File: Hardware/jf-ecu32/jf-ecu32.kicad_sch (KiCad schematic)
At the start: 41 parts, among them J1 GAZ, J10 k, J11 RPM, J12 S.PORT, J2 AUX, J3 PPM/PWM, J4 STARTER, J5 GLOW, J6 VANNE KEROSTART, J7 VANNE KERO, J8 BATTERY 2S/3S, J9 STARTER, Q1 QM6006D, Q2 QM6006D, Q3 QM6006D, Q4 QM6006D, U1 ESP32-DevKitC, U2 4050, U3 MAX31855KASA, U4 AMS1117-3.3, U5 4050

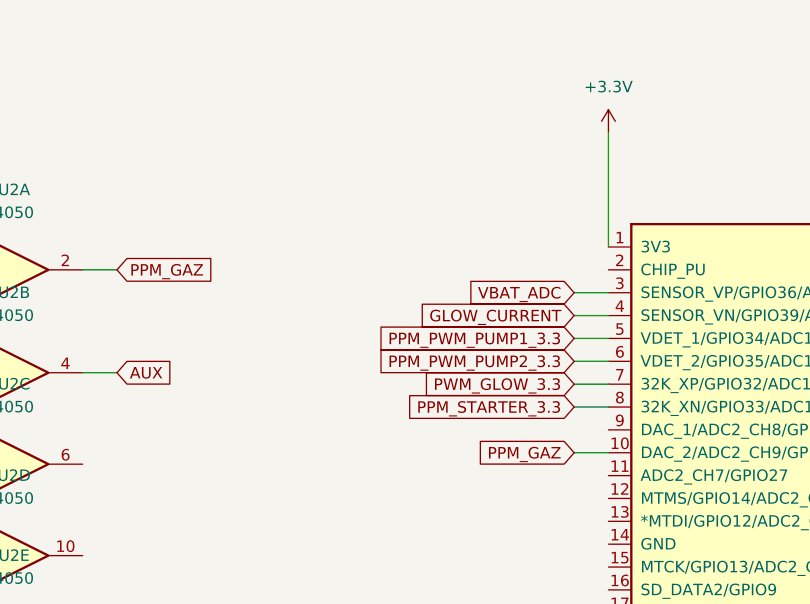
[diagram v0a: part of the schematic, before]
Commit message: update
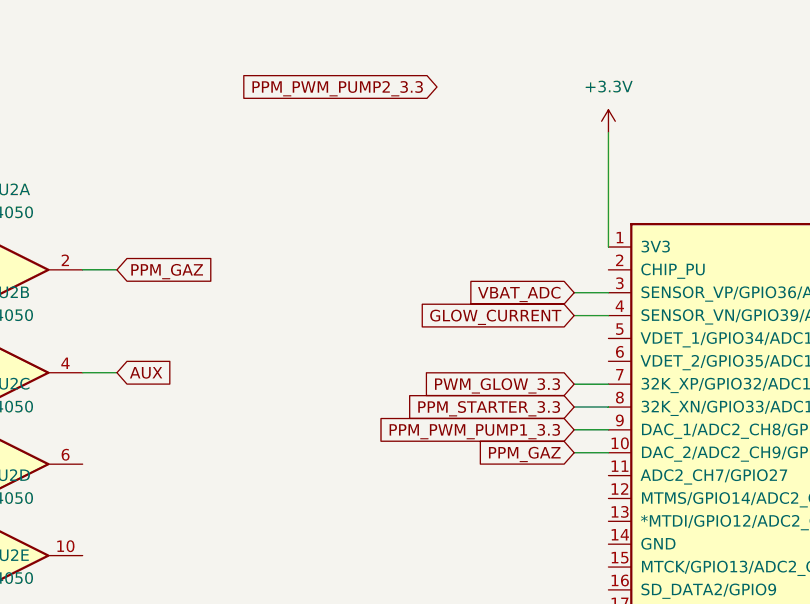
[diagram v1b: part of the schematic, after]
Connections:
- net PPM_PWM_PUMP1_3.3: now also U1.9 (DAC_1/ADC2_CH8/GPIO25); no longer U1.5 (VDET_1/GPIO34/ADC1_CH6)
- net PPM_PWM_PUMP2_3.3: no longer U1.6 (VDET_2/GPIO35/ADC1_CH7)
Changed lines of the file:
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@@
-    (stroke (width 0) (type default) (color 0 0 0 0))
-  )
-  (wire (pts (xy 116.84 53.34) (xy 120.65 53.34))
     (stroke (width 0) (type default) (color 0 0 0 0))
   )
@@
     (stroke (width 0) (type default) (color 0 0 0 0))
   )
+  (wire (pts (xy 116.84 60.96) (xy 120.65 60.96))
+    (stroke (width 0) (type default) (color 0 0 0 0))
+  )
   (wire (pts (xy 382.27 222.25) (xy 384.81 222.25))
     (stroke (width 0) (type default) (color 0 0 0 0))
@@
     (stroke (width 0) (type default) (color 0 0 0 0))
   )
-  (wire (pts (xy 116.84 50.8) (xy 120.65 50.8))
-    (stroke (width 0) (type default) (color 0 0 0 0))
-  )
   (wire (pts (xy 382.27 57.15) (xy 388.62 57.15))
     (stroke (width 0) (type default) (color 0 0 0 0))
@@
     )
   )
-  (global_label "PPM_PWM_PUMP1_3.3" (shape input) (at 116.84 50.8 180) (fields_autoplaced)
-    (effects (font (size 1.27 1.27)) (justify right))
-    (property "Intersheet References" "${INTERSHEET_REFS}" (id 0) (at 93.8045 50.7206 0)
+  (global_label "PPM_PWM_PUMP1_3.3" (shape input) (at 116.84 60.96 180) (fields_autoplaced)
+    (effects (font (size 1.27 1.27)) (justify right))
+    (property "Intersheet References" "${INTERSHEET_REFS}" (id 0) (at 93.8045 60.8806 0)
       (effects (font (size 1.27 1.27)) (justify right) hide)
     )
@@
     )
   )
-  (global_label "PPM_PWM_PUMP2_3.3" (shape input) (at 116.84 53.34 180) (fields_autoplaced)
-    (effects (font (size 1.27 1.27)) (justify right))
-    (property "Intersheet References" "${INTERSHEET_REFS}" (id 0) (at 93.8045 53.2606 0)
-      (effects (font (size 1.27 1.27)) (justify right) hide)
-    )
+  (global_label "PPM_PWM_PUMP2_3.3" (shape input) (at 101.6 22.86 180) (fields_autoplaced)
+    (effects (font (size 1.27 1.27)) (justify right))
+    (property "Intersheet References" "${INTERSHEET_REFS}" (id 0) (at 78.5645 22.7806 0)
+      (effects (font (size 1.27 1.27)) (justify right) hide)
+    )
